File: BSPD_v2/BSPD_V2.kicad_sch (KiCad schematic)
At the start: 13 parts, among them K1 G5V-1, P1 0430450827, T1 T-BJT-NPN, U1 SN74HC00N, U2 LM393P, U3 LM393P, U4 LM393P, U5 SN74HC08N

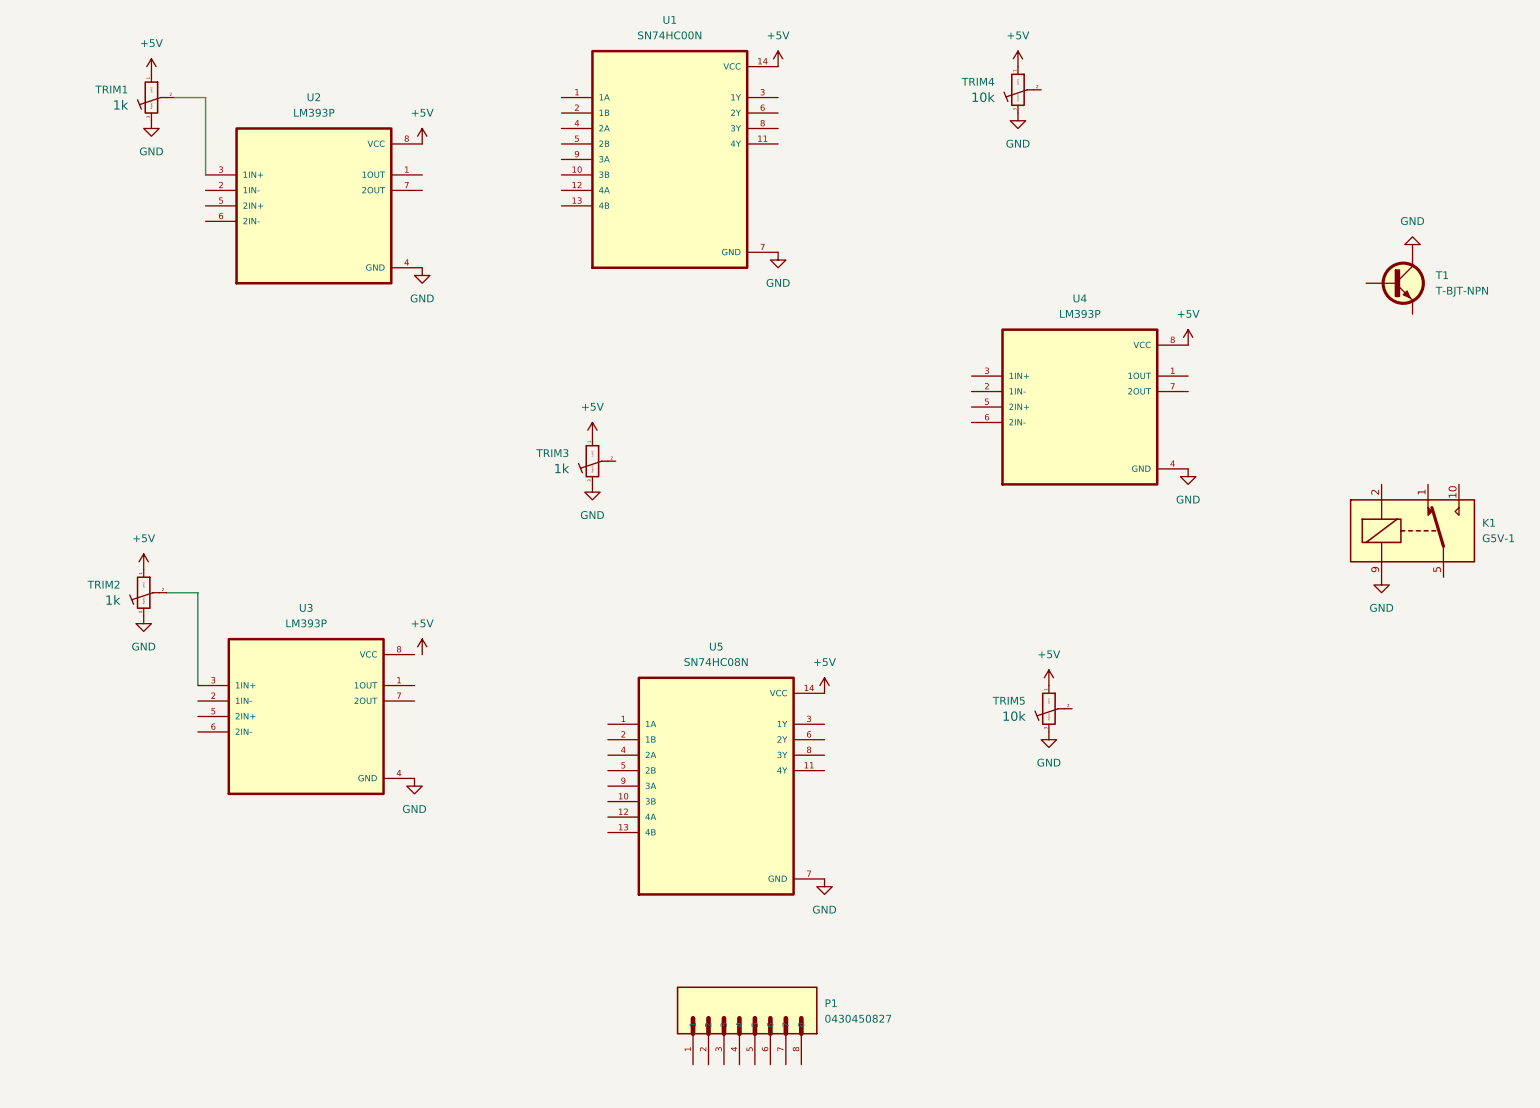
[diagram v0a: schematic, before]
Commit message: updated schematic
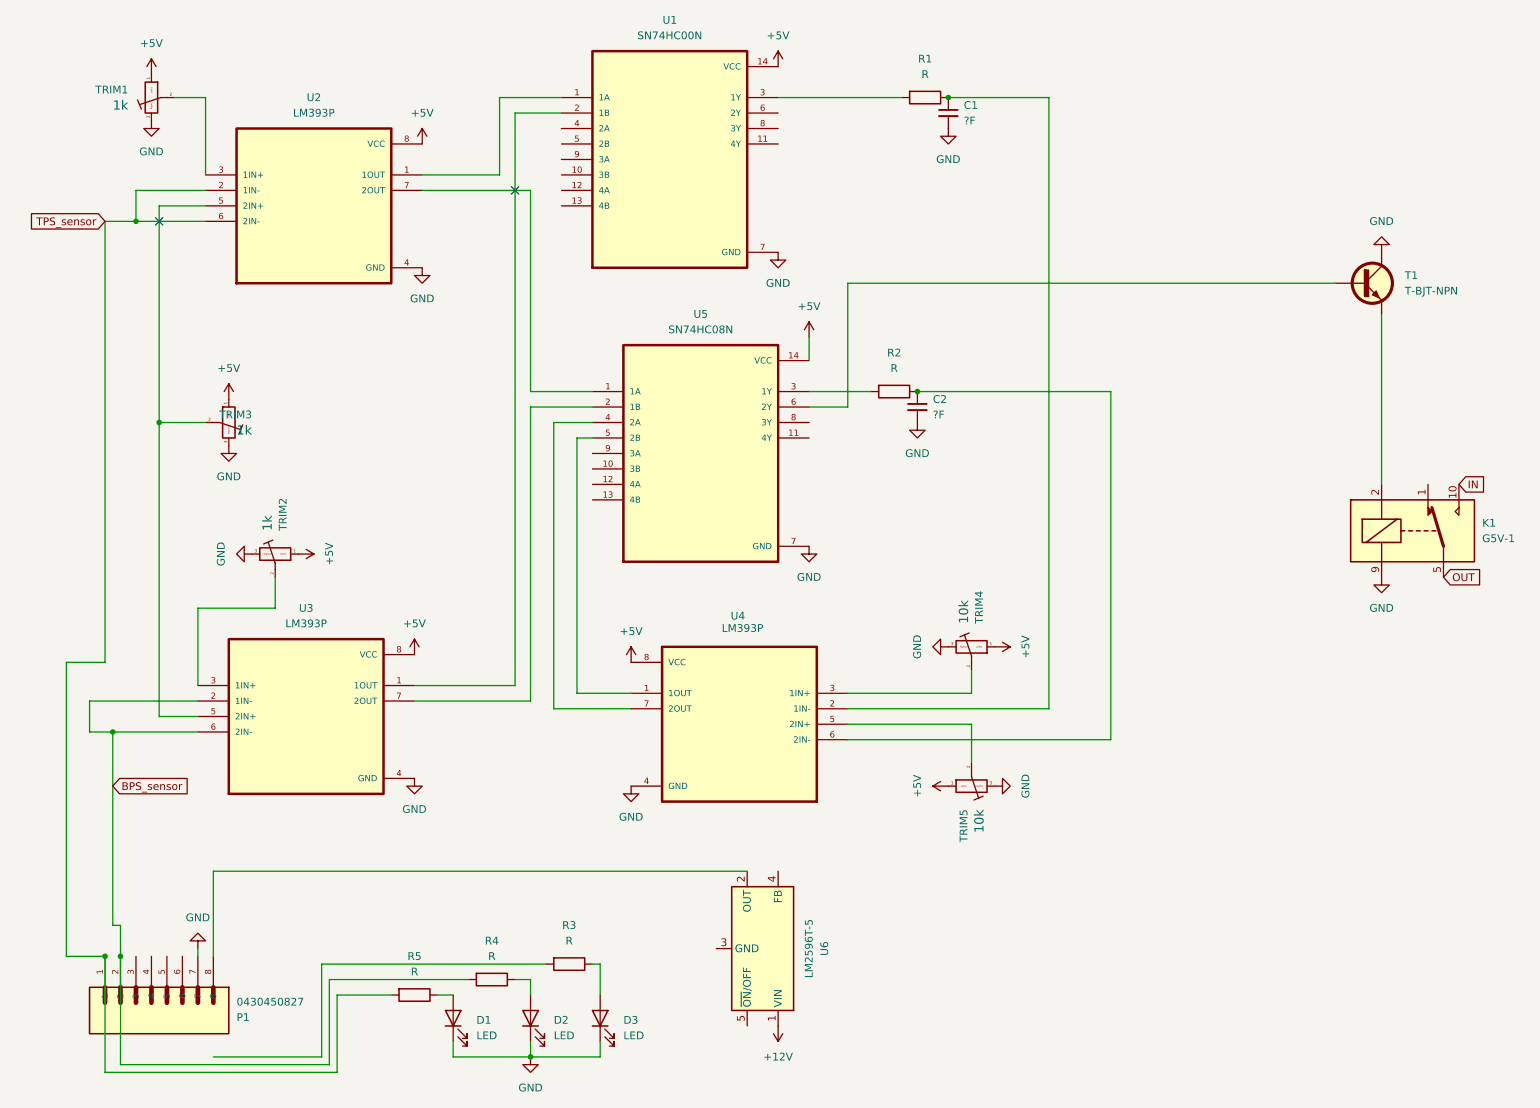
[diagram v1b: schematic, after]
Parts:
- added C1, C2: C_Generic, Capacitor_THT:C_Disc_D12.5mm_W5.0mm_P10.00mm, symbol PCM_4ms_Capacitor:C_Generic
- added D1, D2, D3: LED, LED_THT:LED_D5.0mm_Horizontal_O6.35mm_Z9.0mm, symbol Device:LED
- added R1, R2, R3, R4, R5: R, PCM_Resistor_THT_AKL:R_Axial_DIN0918_L18.0mm_D9.0mm_P25.40mm_Horizontal, symbol Device:R
- added U6: LM2596T-5, PCM_Package_TO_SOT_THT_AKL:TO-220F-5_P3.4x2.06mm_StaggerEven_Lead1.86mm_Vertical, symbol Regulator_Switching:LM2596T-5
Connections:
- net +5V: now also U3.8 (VCC)
- net GND: now also P1.7, C1.2, C2.2, D1.1 (K), D2.1 (K), D3.1 (K)
- net at TRIM4.2 (Center): now also U4.3 (1IN+)
- net at U4.1 (1OUT): now also U5.5 (2B)
- net at U4.2 (1IN-): now also C1.1, R1.1
- net at U4.5 (2IN+): now also TRIM5.2 (Center)
- net at U4.6 (2IN-): now also C2.1, R2.1
- net at U4.7 (2OUT): now also U5.4 (2A)
- net IN: now reaches K1.10
- net at K1.2: now also T1.3 (E)
- net OUT: now reaches K1.5, K1.6
- net at U1.1 (1A): now also U2.1 (1OUT)
- net at U1.2 (1B): now also U3.1 (1OUT)
- net at U1.3 (1Y): now also R1.2
- net BPS_sensor: now reaches U3.2 (1IN-)
- net BPS_sensor: now also P1.2, U3.6 (2IN-), R4.2
- net at U3.5 (2IN+): now also TRIM3.2 (Center), U2.5 (2IN+)
- net at U3.7 (2OUT): now also U5.2 (1B)
- net TPS_sensor: now reaches P1.1
- net TPS_sensor: now also U2.2 (1IN-), U2.6 (2IN-), R5.2
- net at P1.8: now also U6.2 (OUT)
- net at T1.2 (B): now also U5.6 (2Y)
- net at U2.7 (2OUT): now also U5.1 (1A)
- net at U5.3 (1Y): now also R2.2
- new net: D3.2 (A), R3.1
- new net: D2.2 (A), R4.1
- new net: D1.2 (A), R5.1
- new net +12V: U6.1 (VIN)
- no-connect marks 0 -> 2
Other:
- moved on the sheet: P1, T1, TRIM2, TRIM3, TRIM4, TRIM5, U4, U5
